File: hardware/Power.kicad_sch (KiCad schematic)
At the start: 18 parts, among them J1 DC, Q1 DMP3099L-7, U1 ADP7142AUJZ-3.3, U2 ADP7142AUJZ-5.0, U3 ADP7142AUJZ-2.5

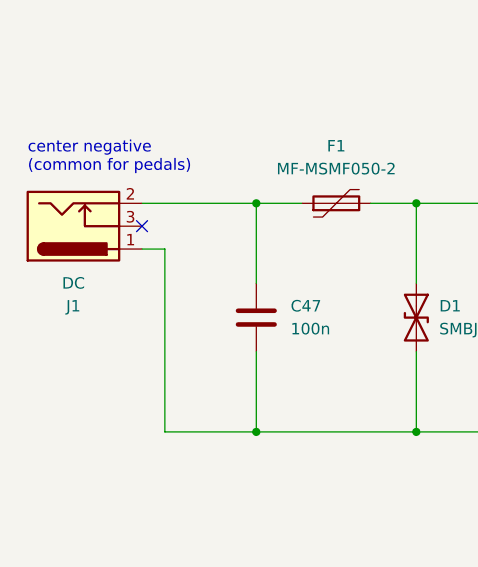
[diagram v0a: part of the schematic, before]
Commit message: added mouser part numbers
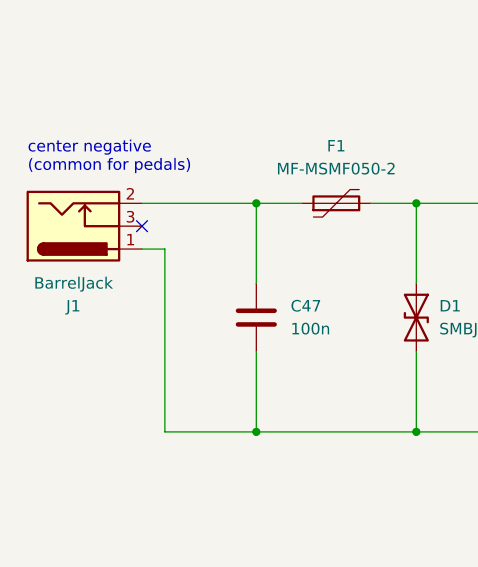
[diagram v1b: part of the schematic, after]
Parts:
- C1: Mouser No (none) -> 667-EEH-ZC1E470P; Part Source (none) -> Mouser
- C2: Notes (none) -> im Uni-Sortiment?; Part Source (none) -> Uni
- C3, C4, C47, C5, C6, C8, R1: Part Source (none) -> Uni
- D1: Mouser No (none) -> 947-SMBJ15CA; Part Source (none) -> Mouser
- D2: Mouser No (none) -> 621-BZX84C15-F; Part Source (none) -> Mouser
- D3: Mouser No (none) -> 771-PMEG6010ELRX; Part Source (none) -> Mouser
- F1: Mouser No (none) -> 652-MF-MSMF050-2; Part Source (none) -> Mouser
- J1: value DC -> BarrelJack; Mouser No (none) -> 490-PJ-102AH; Part Source (none) -> Mouser
- Q1: Mouser No (none) -> 621-DMP3099L-7; Part Source (none) -> Mouser
- U1: Mouser No (none) -> 584-ADP7142AUJZ3.3R7; Part Source (none) -> Mouser
- U2: Mouser No (none) -> 584-ADP7142WAUJZ-50R; Part Source (none) -> Mouser
- U3: Mouser No (none) -> 584-ADP7142AUJZ2.5R7; Part Source (none) -> Mouser
